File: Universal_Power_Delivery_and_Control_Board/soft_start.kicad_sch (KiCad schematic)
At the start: 5 parts, among them Q1 AO4407A, Q3 AO3401A

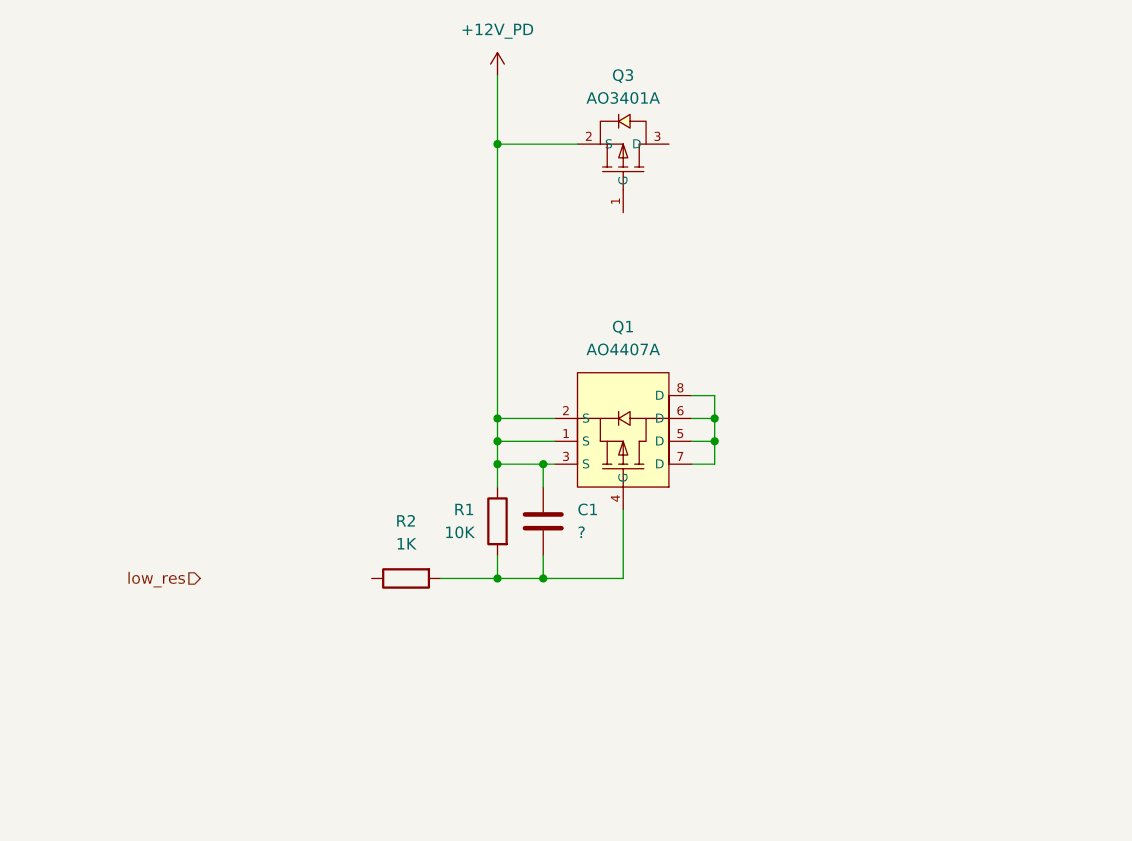
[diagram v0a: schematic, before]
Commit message: Finally figured out the soft start circuitry.
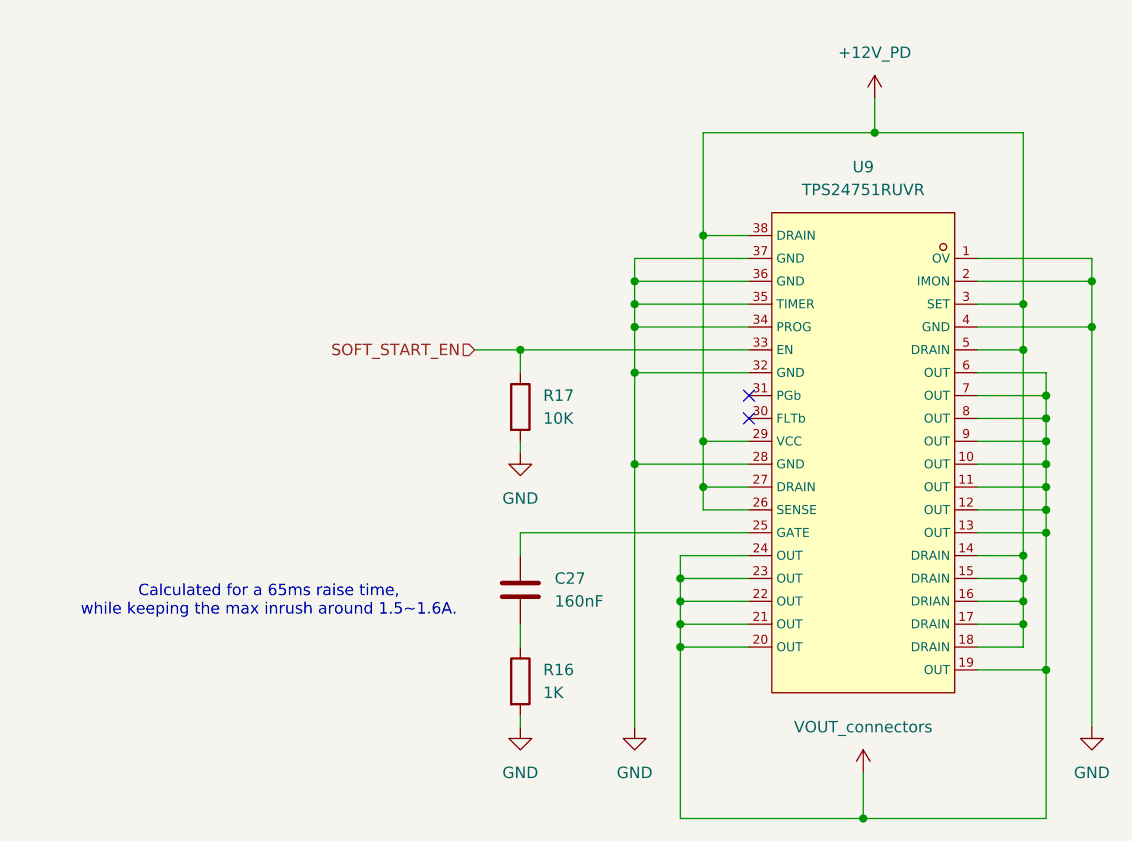
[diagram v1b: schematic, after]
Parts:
- removed C1: ?, Capacitor_SMD:C_0402_1005Metric_Pad0.74x0.62mm_HandSolder, symbol Device:C
- removed Q1: AO4407A, lcsc_footprints:C16072_SOIC-8_L4_9-W3_9-P1_27-LS6_0-BL, symbol lcsc_imported:AO4407A
- removed Q3: AO3401A, lcsc_footprints:C15127_SOT-23_L2_9-W1_3-P1_90-LS2_4-BR, symbol lcsc_imported:AO3401A
- removed R1: 10K, Resistor_SMD:R_0402_1005Metric_Pad0.72x0.64mm_HandSolder, symbol Device:R
- removed R2: 1K, Resistor_SMD:R_0402_1005Metric_Pad0.72x0.64mm_HandSolder, symbol Device:R
- added C27: 160nF, Capacitor_SMD:C_0402_1005Metric_Pad0.74x0.62mm_HandSolder, symbol Device:C
- added R16: 1K, Resistor_SMD:R_0402_1005Metric_Pad0.72x0.64mm_HandSolder, symbol Device:R
- added R17: 10K, Resistor_SMD:R_0402_1005Metric_Pad0.72x0.64mm_HandSolder, symbol Device:R
- added U9: TPS24751RUVR, lcsc_footprints:C2653596_VQFN-36_L7_0-W3_5-P0_50-BL-EP, symbol lcsc_imported:TPS24751RUVR
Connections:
- net +12V_PD: now also U9.14 (DRAIN), U9.15 (DRAIN), U9.16 (DRIAN), U9.17 (DRAIN), U9.18 (DRAIN), U9.26 (SENSE), U9.27 (DRAIN), U9.29 (VCC), U9.3 (SET), U9.38 (DRAIN), U9.5 (DRAIN)
- new net: C27.1, U9.25 (GATE)
- new net: C27.2, R16.1
- new net GND: R16.2, R17.2, U9.1 (OV), U9.2 (IMON), U9.28 (GND), U9.32 (GND), U9.34 (PROG), U9.35 (TIMER), U9.36 (GND), U9.37 (GND), U9.4 (GND)
- new net SOFT_START_EN: R17.1, U9.33 (EN)
- new net VOUT_connectors: U9.10 (OUT), U9.11 (OUT), U9.12 (OUT), U9.13 (OUT), U9.19 (OUT), U9.20 (OUT), U9.21 (OUT), U9.22 (OUT), U9.23 (OUT), U9.24 (OUT), U9.6 (OUT), U9.7 (OUT), U9.8 (OUT), U9.9 (OUT)
- no-connect marks 0 -> 2
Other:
- note added: "Calculated for a 65ms raise time, while keeping the max inrush around 1.5~1.6A."
